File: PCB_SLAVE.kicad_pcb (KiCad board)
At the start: 2 copper layers, 88.7 x 70 mm, 44 parts, among them J1 RGB, J10 DHT, J2 Conn_01x03, J3 MOTOR_DC, J4 LED_OUT, J7 MOTOR, J8 zigbee, J9 DAT, K1 G5LE-1, Q1 2SC1815, Q2 IRF540N, Q3 2SC1815, SW1 SW_Push, SW2 SW_Push, SW3 SW_Push, U1 PC817, U2 LM2576HVS-AJD

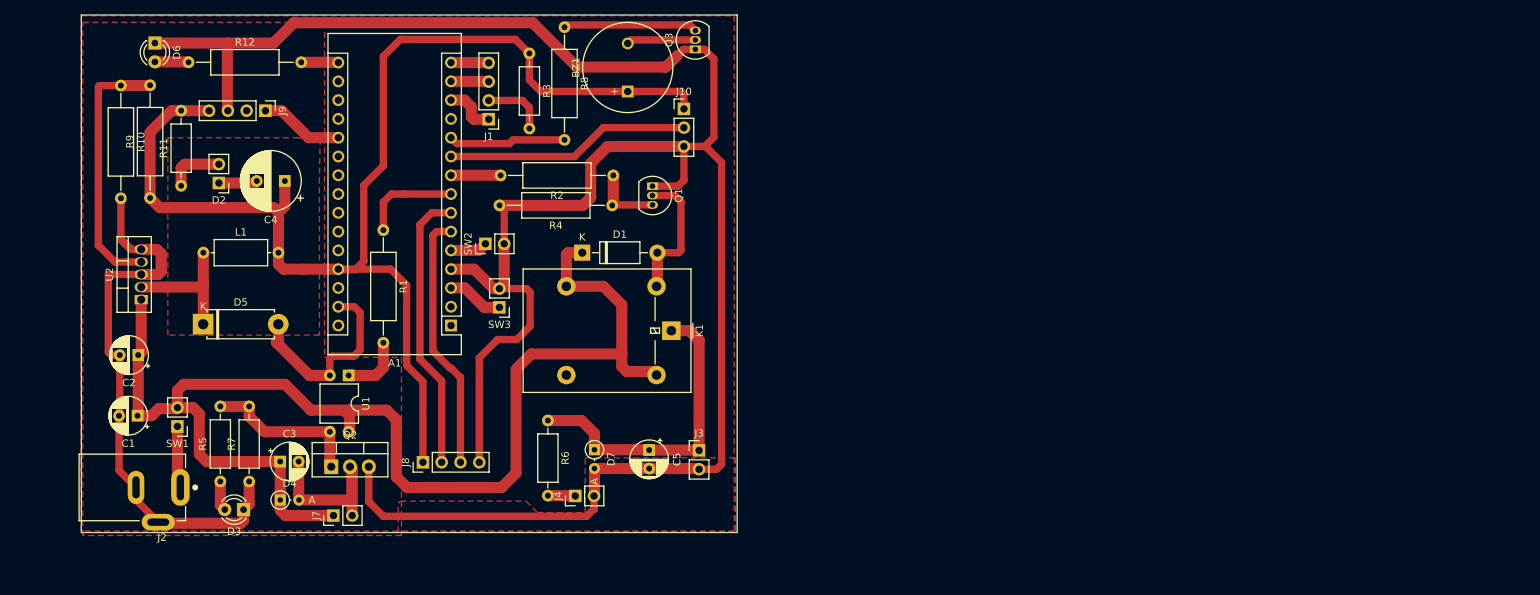
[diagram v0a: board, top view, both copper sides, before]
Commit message: add file
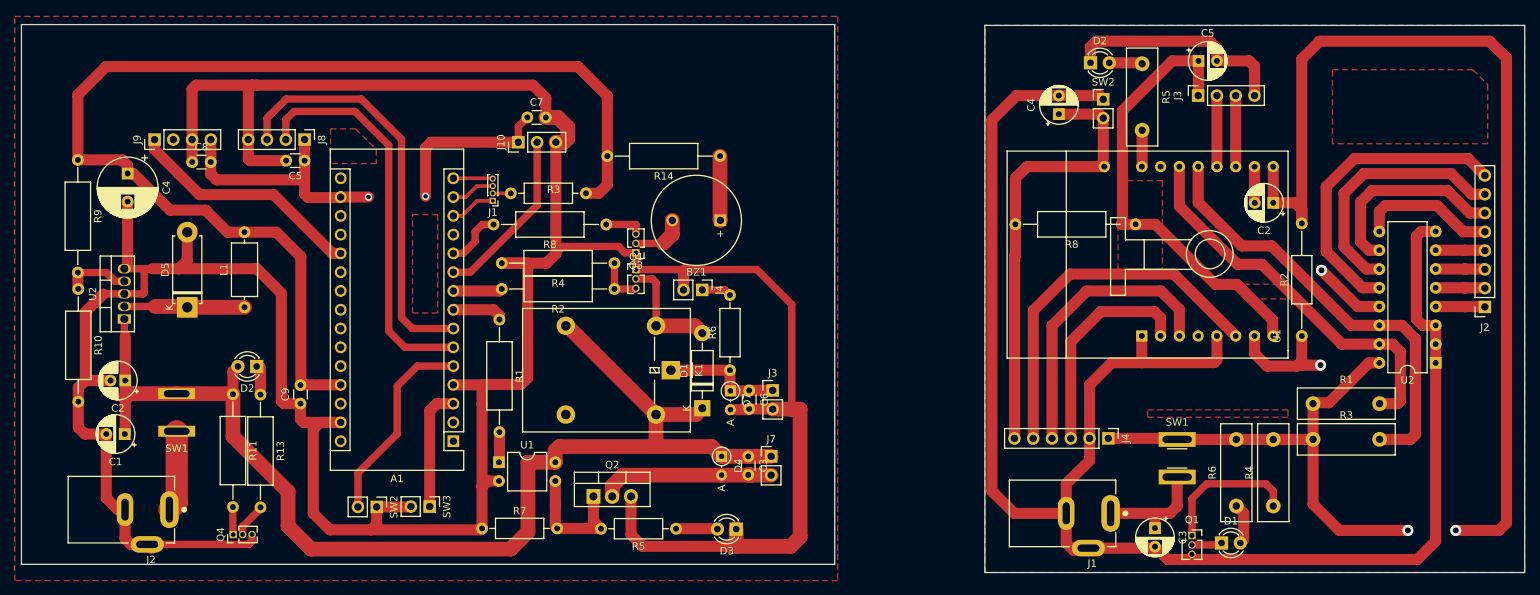
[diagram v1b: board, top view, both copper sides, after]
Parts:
- removed the C2 at (41.1, 63.9)
- removed the C3 at (60.3, 78.3)
- removed the C4 at (60.9, 40.4)
- removed the C5 at (110.2, 76.8)
- removed the D1 at (101.2, 50.0)
- removed the D2 at (52.0, 40.6)
- removed D6: LED_Small, LED_THT:LED_D3.0mm
- removed the J1 at (88.5, 32.0)
- removed the J2 at (46.8, 81.8)
- removed the J3 at (117.0, 76.8)
- removed the J4 at (100.2, 83.0)
- removed the Q1 at (110.7, 41.0)
- removed the R1 at (74.2, 47.0)
- removed R12: 330, Resistor_THT:R_Axial_DIN0309_L9.0mm_D3.2mm_P15.24mm_Horizontal
- removed the R2 at (105.3, 39.6)
- removed the R3 at (94.0, 23.1)
- removed the R4 at (105.2, 43.6)
- removed the R5 at (52.2, 81.0)
- removed the R6 at (96.5, 72.8)
- removed the R8 at (98.8, 19.6)
- removed the SW1 at (46.4, 73.5)
- removed the SW2 at (88.0, 48.9)
- removed the U1 at (69.5, 66.7)
- removed the U2 at (41.5, 56.4)
- added C2: 104, Capacitor_THT:CP_Radial_D5.0mm_P2.50mm, F.Cu at (194.6, 43.3)
- added C2: 10uF, Capacitor_THT:CP_Radial_D5.0mm_P2.00mm, F.Cu at (39.3, 67.3)
- added C3: 104, Capacitor_THT:CP_Radial_D5.0mm_P2.50mm, F.Cu at (178.6, 87.3)
- added C3: 104, Capacitor_THT:C_Disc_D3.0mm_W1.6mm_P2.50mm, F.Cu at (123.6, 77.6)
- added C4: 100nF, Capacitor_THT:CP_Radial_D5.0mm_P2.50mm, F.Cu at (165.6, 31.3)
- added C4: 1000uF, Capacitor_THT:CP_Radial_D8.0mm_P3.80mm, F.Cu at (39.7, 39.3)
- added C5: 104, Capacitor_THT:CP_Radial_D5.0mm_P2.50mm, F.Cu at (184.5, 24.1)
- added C5: 104, Capacitor_THT:C_Disc_D3.0mm_W1.6mm_P2.50mm, F.Cu at (63.6, 37.6)
- added C6: 104, Capacitor_THT:C_Disc_D3.0mm_W1.6mm_P2.50mm, F.Cu at (123.7, 68.7)
- added C7: 104, Capacitor_THT:C_Disc_D3.0mm_W1.6mm_P2.50mm, F.Cu at (93.7, 31.8)
- added C8: 104, Capacitor_THT:C_Disc_D3.0mm_W1.6mm_P2.50mm, F.Cu at (48.4, 37.8)
- added C9: 104, Capacitor_THT:C_Disc_D3.0mm_W1.6mm_P2.50mm, F.Cu at (63.0, 70.5)
- added D1: LED_Small, LED_THT:LED_D3.0mm, F.Cu at (187.6, 89.3)
- added D1: 1N4148, Diode_THT:D_DO-41_SOD81_P10.16mm_Horizontal, F.Cu at (117.4, 71.1)
- added D2: LED_Small, LED_THT:LED_D3.0mm, F.Cu at (169.9, 24.4)
- added D2: LED_Nguon, LED_THT:LED_D3.0mm, F.Cu at (57.1, 65.4)
- added J1: Power_5V, FOOTRINF:jack_DC, F.Cu at (172.6, 85.3)
- added J1: RGB, Connector_PinHeader_1.00mm:PinHeader_1x04_P1.00mm_Vertical, F.Cu at (89.0, 43.0)
- added J2: OUT, Connector_PinSocket_2.54mm:PinSocket_1x08_P2.54mm_Vertical, F.Cu at (223.2, 57.4)
- added J2: POWER _ 12V, jack_dc:jack_DC, F.Cu at (45.3, 84.8)
- added J3: ZIGBEE, Connector_PinSocket_2.54mm:PinSocket_1x04_P2.54mm_Vertical, F.Cu at (184.5, 28.8)
- added J3: MOTOR_DC, Connector_PinHeader_2.54mm:PinHeader_1x02_P2.54mm_Vertical, F.Cu at (126.9, 68.7)
- added J4: FLASH, Connector_PinHeader_2.54mm:PinHeader_1x06_P2.54mm_Vertical, F.Cu at (172.3, 75.2)
- added J4: LED_TUOI, Connector_PinHeader_2.54mm:PinHeader_1x02_P2.54mm_Vertical, F.Cu at (117.4, 55.1)
- added Q1: Q_NPN_BCE, Connector_PinSocket_1.27mm:PinSocket_1x03_P1.27mm_Vertical, F.Cu at (183.6, 88.3)
- added Q1: 2SC1815, Connector_PinHeader_1.27mm:PinHeader_1x03_P1.27mm_Vertical, F.Cu at (108.4, 52.3)
- added Q4: 2SC1815, Connector_PinHeader_1.27mm:PinHeader_1x03_P1.27mm_Vertical, F.Cu at (53.9, 88.2)
- added R1: 4.7K, Resistor_THT:R_Box_L13.0mm_W4.0mm_P9.00mm, F.Cu at (200.0, 70.5)
- added R1: 220, Resistor_THT:R_Axial_DIN0309_L9.0mm_D3.2mm_P15.24mm_Horizontal, F.Cu at (90.0, 59.1)
- added R13: 470, Resistor_THT:R_Axial_DIN0309_L9.0mm_D3.2mm_P15.24mm_Horizontal, F.Cu at (57.6, 69.2)
- added R14: 10R, Resistor_THT:R_Axial_DIN0309_L9.0mm_D3.2mm_P15.24mm_Horizontal, F.Cu at (119.8, 37.0)
- added R2: 10K, Resistor_THT:R_Axial_DIN0207_L6.3mm_D2.5mm_P15.24mm_Horizontal, F.Cu at (198.5, 61.3)
- added R2: 100, Resistor_THT:R_Axial_DIN0309_L9.0mm_D3.2mm_P15.24mm_Horizontal, F.Cu at (105.5, 55.0)
- added R3: 4.7K, Resistor_THT:R_Box_L13.0mm_W4.0mm_P9.00mm, F.Cu at (200.0, 75.3)
- added R3: 220, Resistor_THT:R_Axial_DIN0207_L6.3mm_D2.5mm_P10.16mm_Horizontal, F.Cu at (101.6, 42.0)
- added R4: 1K, Resistor_THT:R_Box_L13.0mm_W4.0mm_P9.00mm, F.Cu at (194.6, 84.3)
- added R4: 10K, Resistor_THT:R_Axial_DIN0309_L9.0mm_D3.2mm_P15.24mm_Horizontal, F.Cu at (105.5, 51.5)
- added R5: 220, Resistor_THT:R_Box_L13.0mm_W4.0mm_P9.00mm, F.Cu at (176.9, 24.5)
- added R5: 470, Resistor_THT:R_Axial_DIN0207_L6.3mm_D2.5mm_P10.16mm_Horizontal, F.Cu at (113.8, 87.4)
- added R6: 220, Resistor_THT:R_Box_L13.0mm_W4.0mm_P9.00mm, F.Cu at (189.6, 84.3)
- added R6: 470, Resistor_THT:R_Axial_DIN0207_L6.3mm_D2.5mm_P10.16mm_Horizontal, F.Cu at (121.1, 65.9)
- added R8: 10K, Resistor_THT:R_Axial_DIN0309_L9.0mm_D3.2mm_P15.24mm_Horizontal, F.Cu at (175.0, 46.2)
- added R8: 1K, Resistor_THT:R_Axial_DIN0309_L9.0mm_D3.2mm_P15.24mm_Horizontal, F.Cu at (104.4, 46.2)
- added SW1: SW_Push, Connector_PinHeader_2.54mm:PinHeader_1x02_P2.54mm_Vertical, F.Cu at (181.6, 75.3)
- added SW1: NGUON, Connector_PinHeader_2.54mm:PinHeader_1x02_P2.54mm_Vertical, F.Cu at (46.3, 74.2)
- added SW2: SW_Push, Connector_PinHeader_2.54mm:PinHeader_1x02_P2.54mm_Vertical, F.Cu at (171.6, 29.3)
- added SW2: CLEAR_EPR, Connector_PinHeader_2.54mm:PinHeader_1x02_P2.54mm_Vertical, F.Cu at (73.4, 84.4)
- added U1: ESP32_AI_THINKER, FOOTRINF:ESP_CAM, F.Cu at (194.6, 61.3)
- added U1: PC817, Package_DIP:DIP-4_W7.62mm, F.Cu at (89.9, 78.4)
- added U2: PCF8574A, Package_DIP:DIP-16_W7.62mm, F.Cu at (216.6, 65.0)
- added U2: LM2576HVS-AJD, Package_TO_SOT_THT:TO-220-5_Vertical, F.Cu at (39.2, 59.0)
- D3: value LED_Small -> LED_PHUN
- D4, D7: value 1N4008 -> 1N4148
- Q3: footprint Package_TO_SOT_THT:TO-92_Inline -> Connector_PinHeader_1.27mm:PinHeader_1x03_P1.27mm_Vertical
- R11: footprint Resistor_THT:R_Axial_DIN0207_L6.3mm_D2.5mm_P10.16mm_Horizontal -> Resistor_THT:R_Axial_DIN0309_L9.0mm_D3.2mm_P15.24mm_Horizontal
- SW3: value SW_Push -> RST
- moved D3 66.7 mm to (122.0, 87.4)
- moved D4 60.0 mm to (120.0, 77.6), turned to 270 degrees
- moved J7 59.7 mm to (126.7, 77.6), turned to 0 degrees
- moved J8 46.5 mm to (63.6, 34.8), turned to 270 degrees
- moved Q2 35.7 mm to (102.7, 83.0)
- moved R7 32.1 mm to (87.6, 87.3), turned to 0 degrees
- moved R11 29.1 mm to (53.9, 69.2), turned to 270 degrees
- moved Q3 28.7 mm to (108.4, 50.1), turned to 180 degrees
- moved SW3 28.5 mm to (80.5, 84.4), turned to 270 degrees
- moved R10 28.1 mm to (33.0, 55.0)
- moved J10 22.8 mm to (92.5, 35.1), turned to 90 degrees
- moved BZ1 21.5 mm to (119.8, 45.7), turned to 180 degrees
- moved D7 20.0 mm to (121.2, 68.7)
- moved A1 15.7 mm to (83.7, 75.5)
- moved J9 15.5 mm to (43.3, 34.8), turned to 90 degrees
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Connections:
- A1 pad 17: Net-(A1-Pad17) -> +3V3
- A1 pad 5: CLEAR_EPR -> Net-(A1-Pad5)
- A1 pad 6: ZIG_RX -> ZIG_TX
- A1 pad 7: ZIG_TX -> ZIG_RX
- BZ1 pad 1: +5V -> Net-(BZ1-Pad1)
- J10 pad 1: +5V -> +3V3
- J8 pad 1: +5V -> +3V3
- J9 pad 4: +5V -> +3V3
- R11 pad 1: Net-(D2-Pad2) -> +12V
- R11 pad 2: +5V -> Net-(Q4-Pad1)
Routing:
- net (no net): track 0.00 -> 1069.1 mm, vias 0 -> 5
- net +3V3: track 0.00 -> 57.2 mm, vias 0 -> 2
- net +12V: track 215.0 -> 162.9 mm
- net Net-(A1-Pad5): track 0.00 -> 27.3 mm
- net Net-(C6-Pad1): track 43.5 -> 16.6 mm
- net Net-(R10-Pad1): track 35.3 -> 9.03 mm
- net ZIG_RX: track 35.0 -> 56.9 mm
- net A1: track 11.4 -> 32.3 mm
- net ZIG_TX: track 38.2 -> 53.8 mm
- net +5V: track 172.9 -> 158.1 mm
- net Net-(Q3-Pad3): track 18.1 -> 5.28 mm
- net SIG_DHT: track 33.1 -> 23.6 mm
- net Net-(C3-Pad2): track 33.5 -> 24.2 mm
- net Net-(A1-Pad3): track 7.68 -> 16.6 mm
- net Net-(BZ1-Pad1): track 0.00 -> 8.71 mm
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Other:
- board size 88.7 x 70 mm -> 203.3 x 74.1 mm
